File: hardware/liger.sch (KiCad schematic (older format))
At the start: 54 parts, among them P1 CONN_01X10, P2 CONN_01X10, P4 CONN_01X02, P5 CONN_01X04, Q1 Q_NMOS_GSD, Q2 Q_PMOS_GSD, Q3 Q_NPN_BEC, Q4 Q_NPN_BEC, SW1 SW_PUSH, U11 SPX3819, U2 ADA4075, U3 ESP-WROOM-02, U5 PT5529B/L2/H2-F

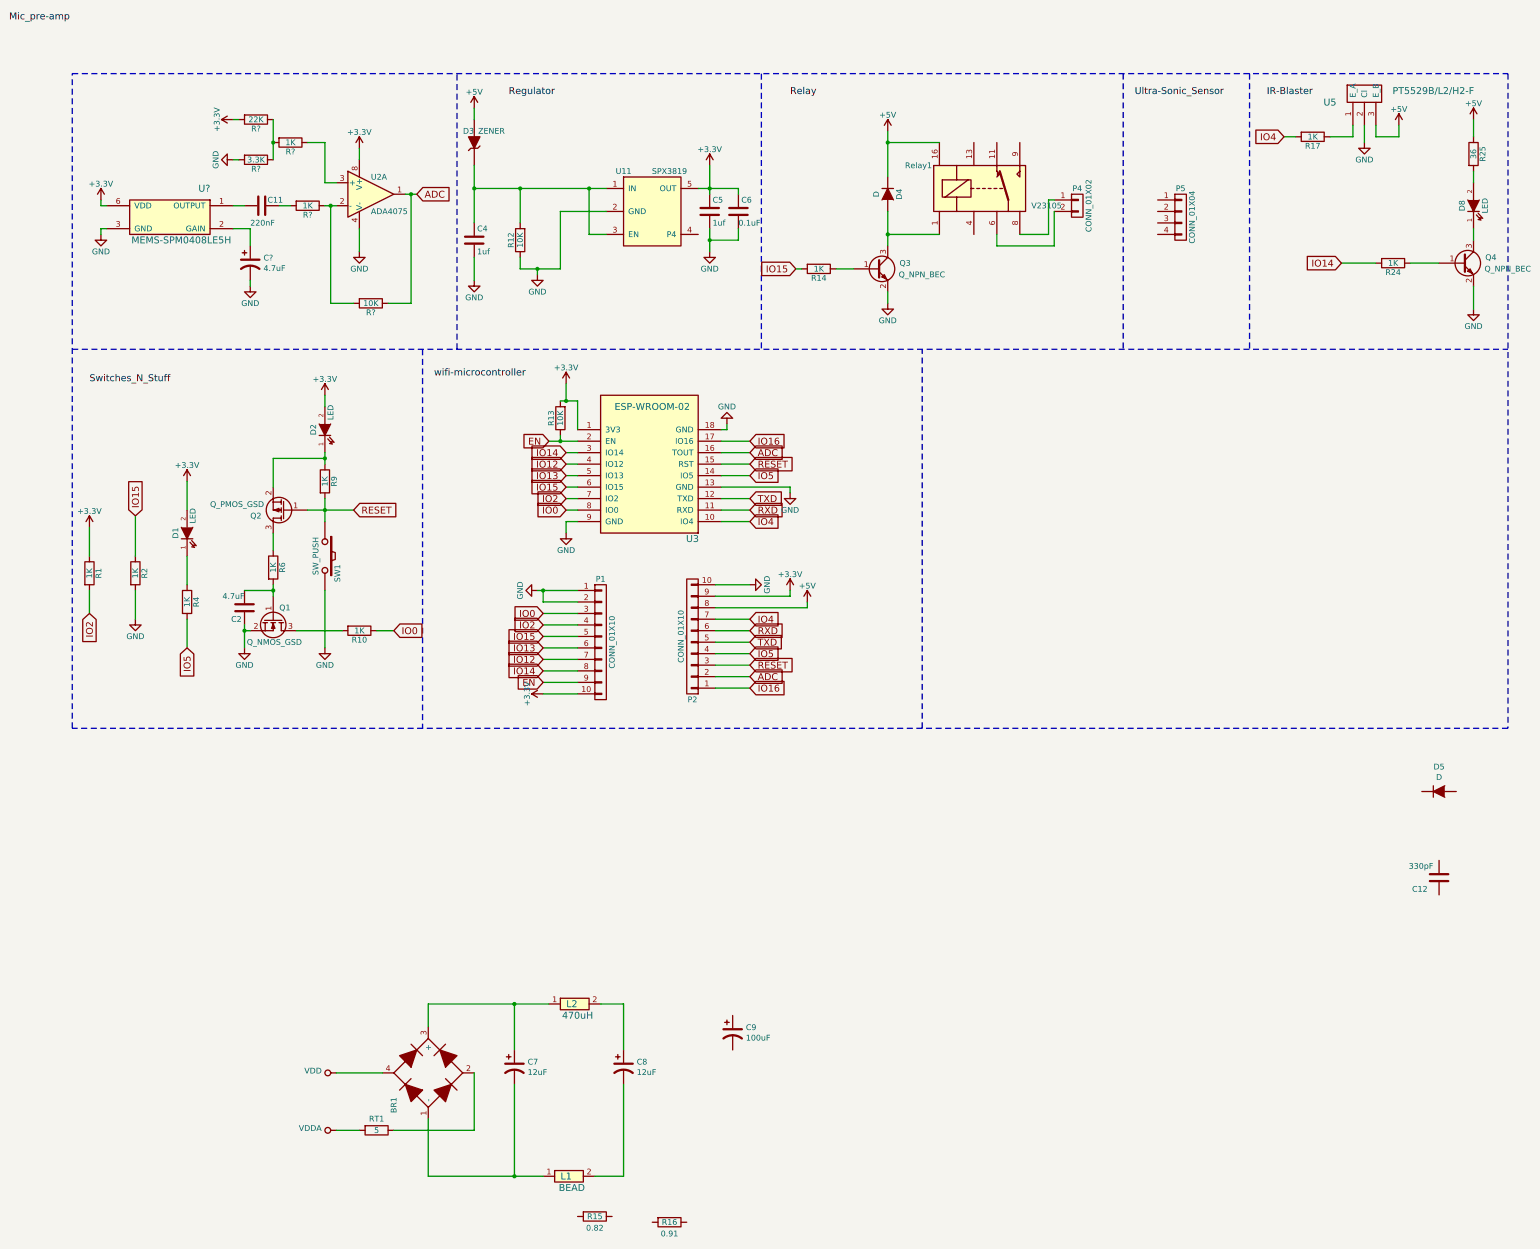
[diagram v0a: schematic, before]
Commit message: update
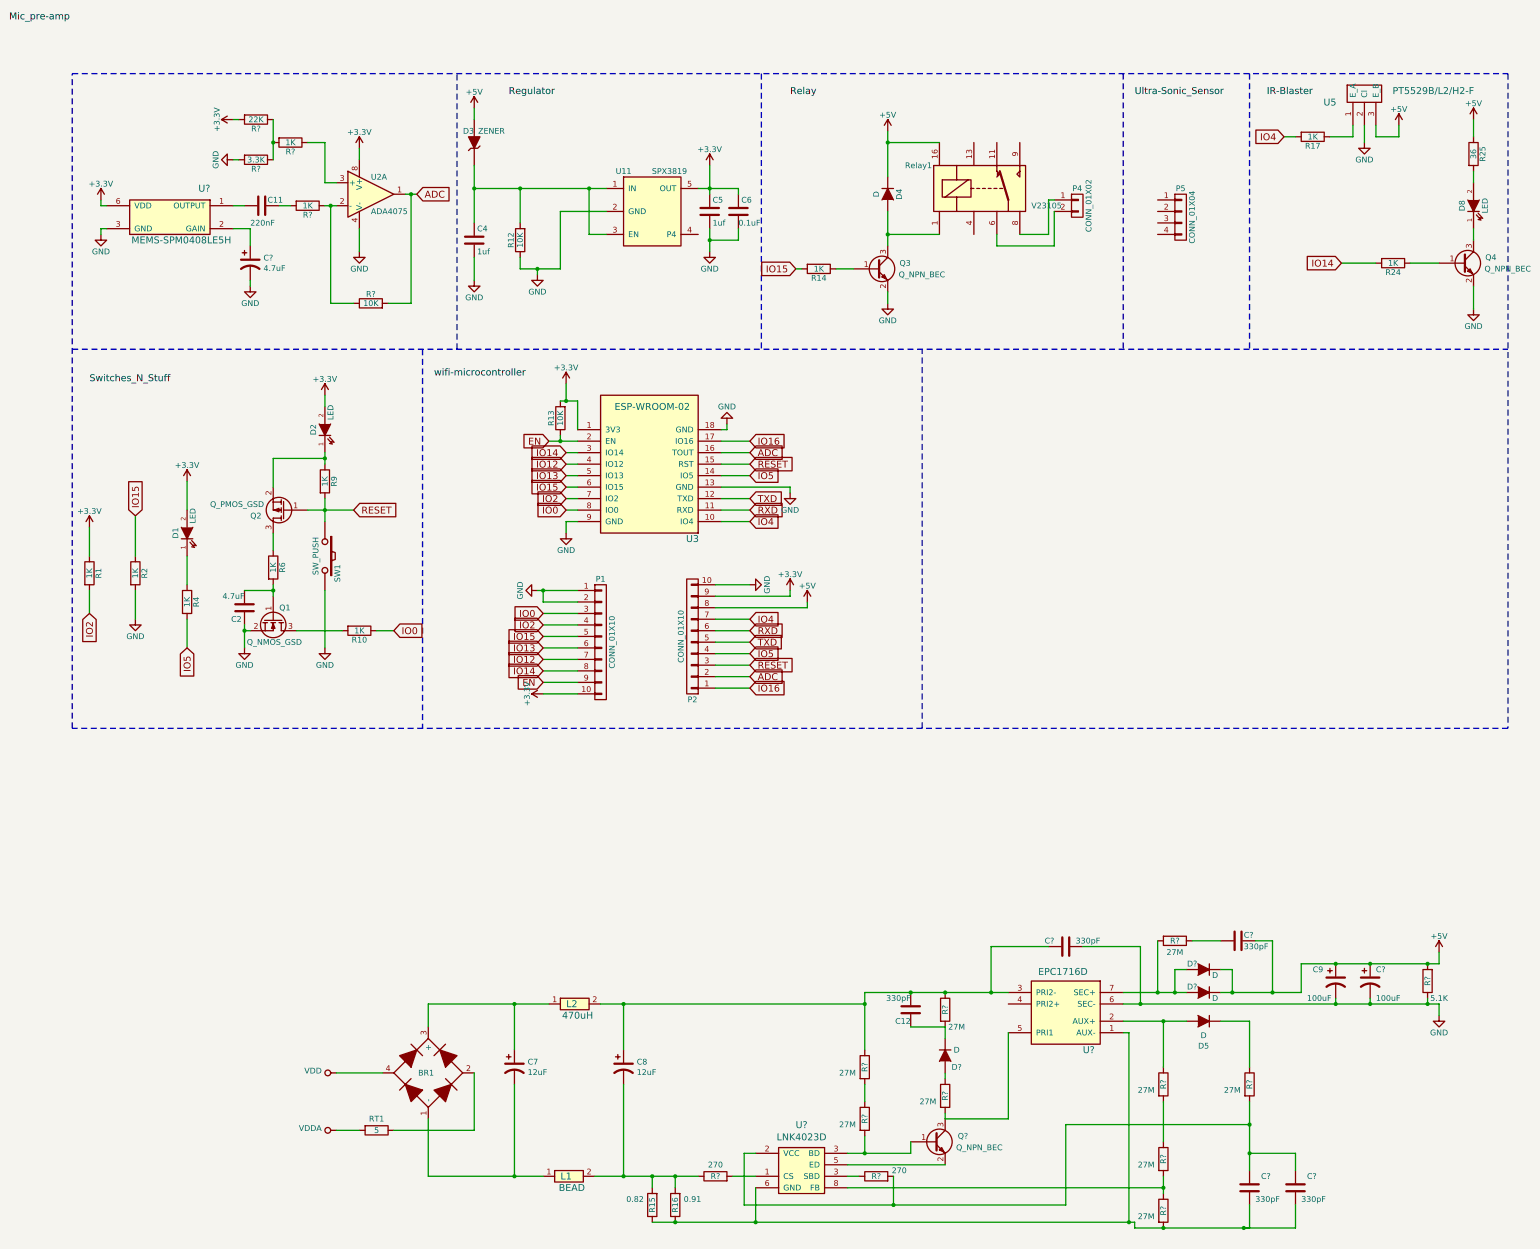
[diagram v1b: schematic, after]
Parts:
- removed R? (x2): 1K, Resistors_SMD:R_0603, symbol R
- removed R?: 10K, Resistors_SMD:R_0603, symbol R
- added C? (x4): 330pF, Capacitors_SMD:C_0805_HandSoldering, symbol C
- added C?: 100uF, Capacitors_ThroughHole:C_Radial_D10_L20_P7.5, symbol CP1
- added D? (x3): D, Diodes_SMD:SMB_Handsoldering, symbol D
- added Q?: Q_NPN_BEC, TO_SOT_Packages_SMD:SOT-23, symbol Q_NPN_BEC
- added R? (x2): 1K, Resistors_SMD:R_0603, symbol R
- added R?: 10K, Resistors_SMD:R_0603, symbol R
- added R? (x2): 270, Resistors_SMD:R_0805_HandSoldering, symbol R
- added R? (x9): 27M, Resistors_SMD:R_0805_HandSoldering, symbol R
- added R?: 5.1K, Resistors_SMD:R_0805_HandSoldering, symbol R
- added U?: LNK4023D, symbol LNK4023D
- added U?: EPC1716D, symbol EPC1716D
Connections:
- net +5V: now also C9.1, C?.1, C?.1, D?.1 (K), D?.1 (K), R?.2
- net ADC: now also R?.2
- net GND: now also C9.2, C?.2, C?.2, R?.1, U?.6 (SEC-)
- net at U2.2 (-): now also R?.1, R?.1
- net at U2.3 (+): now also R?.1
- net at C12.1: now also D?.1 (K), R?.2
- net at C12.2: now also C8.1, L2.2, C?.1, R?.1, R?.1, U?.3 (PRI2-)
- net at C11.1: now also R?.2
- net at D5.1 (K): now also R?.1
- net at D5.2 (A): now also R?.1, U?.2 (AUX+)
- net at C8.2, L1.2: now also R15.2, R16.2, R?.1
- net at R16.1: now also R15.1, C?.2, C?.2, R?.2, U?.1 (AUX-), U?.6 (GND)
- net at R?.1, R?.1: now also R?.2
- new net: R?.2, U?.1 (CS)
- new net: C?.1, C?.1, R?.2, R?.2, U?.2 (VCC)
- new net: R?.1, U?.3 (SBD)
- new net: Q?.1 (B), R?.2, U?.3 (SBD)
- new net: Q?.2 (E), U?.5 (ED)
- new net: R?.1, R?.2, U?.8 (FB)
- new net: R?.1, R?.2 (x2)
- new net: Q?.3 (C), R?.2, U?.5 (PRI1)
- new net: D?.2 (A), R?.1
- new net: D?.2 (A), D?.2 (A), R?.2, U?.7 (SEC+)
- new net: C?.2, R?.1
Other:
- moved on the sheet: C12, C9, D5, R15, R16
